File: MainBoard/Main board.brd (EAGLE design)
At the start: 100 x 80 mm, 9 parts

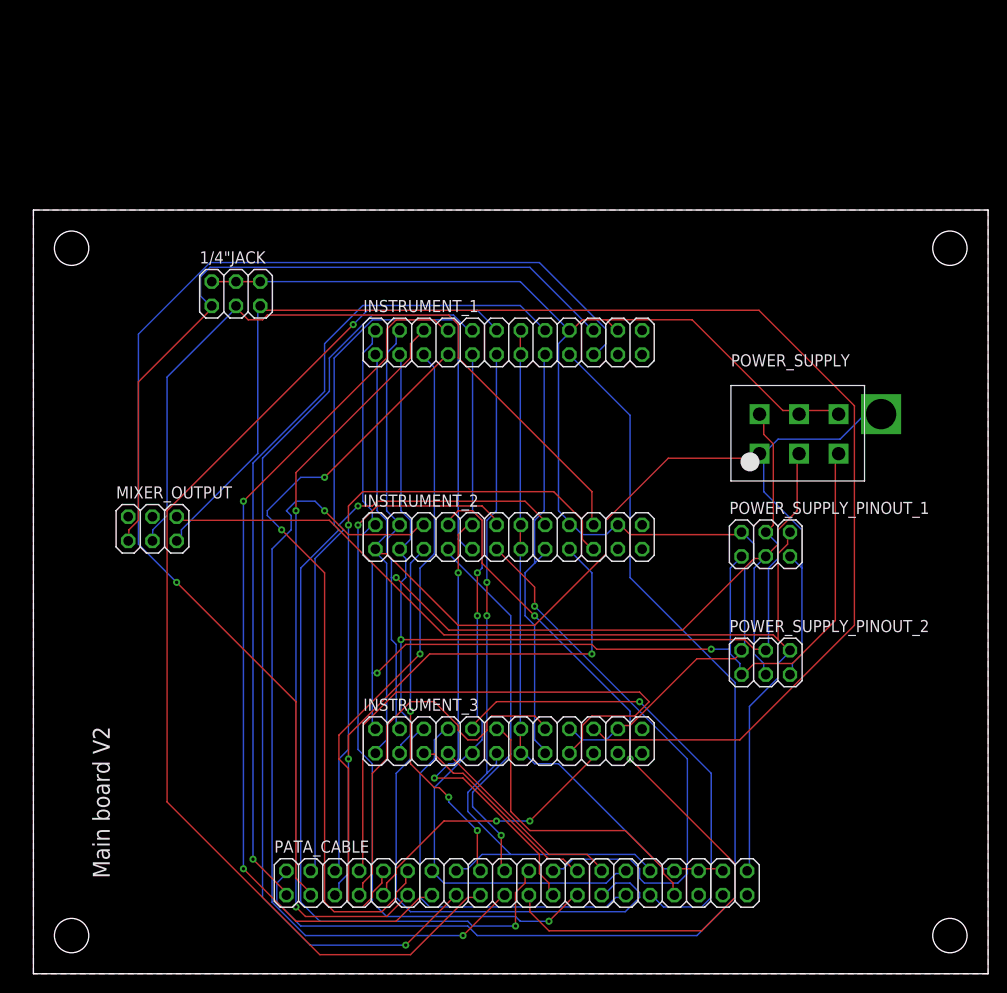
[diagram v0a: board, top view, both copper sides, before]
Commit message: Finished layout - needs silk screen
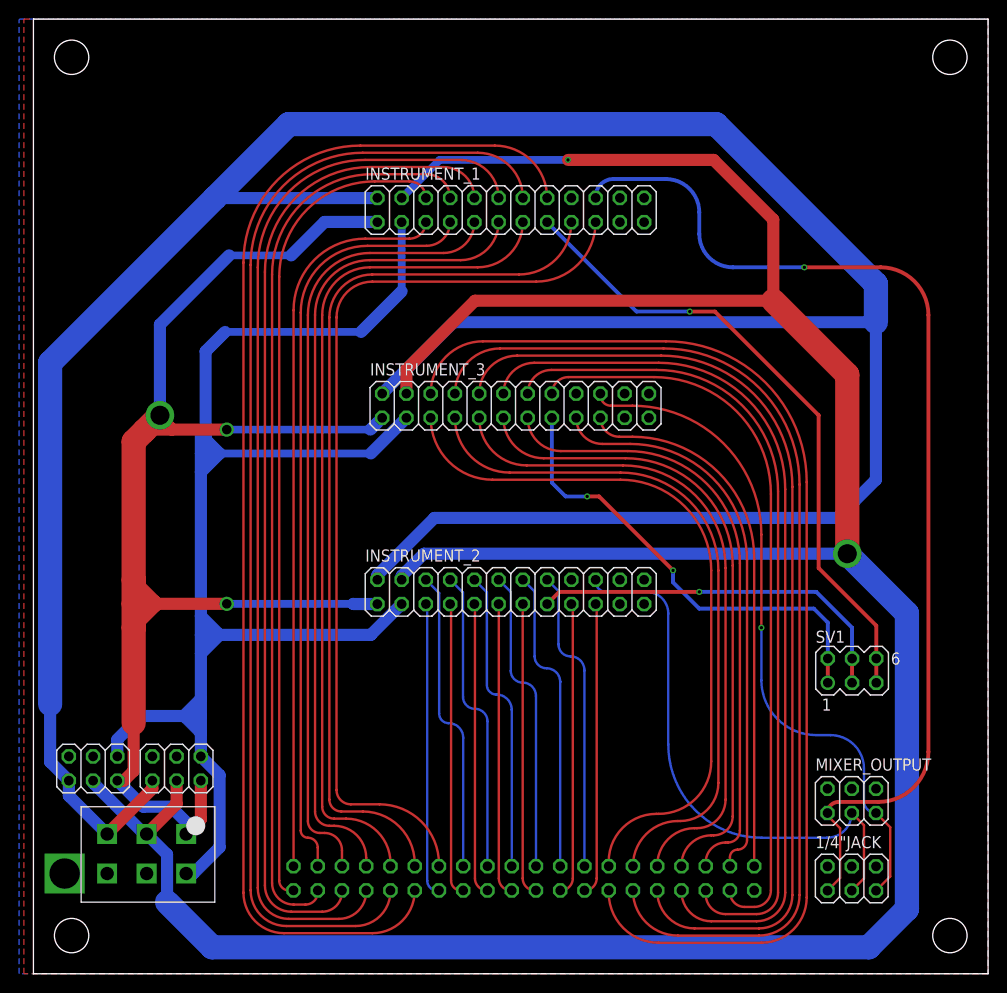
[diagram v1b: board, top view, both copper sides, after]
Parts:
- added SV1: (no value), con-lstb:MA03-2
- moved 1/4"JACK 88.9 mm to (85.7, 9.98)
- moved MIXER_OUTPUT 78.6 mm to (85.7, 18.1)
- moved POWER_SUPPLY 77.0 mm to (16.0, 10.5), turned to 180 degrees
- moved POWER_SUPPLY_PINOUT_1 74.3 mm to (6.25, 21.5)
- moved POWER_SUPPLY_PINOUT_2 62.7 mm to (15.0, 21.5)
- moved INSTRUMENT_3 35.1 mm to (50.5, 59.5)
- moved INSTRUMENT_1 13.9 mm to (50.0, 80.0)
- moved INSTRUMENT_2 5.75 mm to (50.0, 40.0)
- moved PATA_CABLE 0.89 mm to (51.4, 10.0), flipped to the bottom, turned to 180 degrees
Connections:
- net ANALOG_OUTPUT_1 renamed OUT1
- net ANALOG_OUTPUT_2 renamed OUT2
- net ANALOG_OUTPUT_3 renamed OUT3
- removed net ANALOG_GND: 1/4"JACK.2, 1/4"JACK.4, 1/4"JACK.6, INSTRUMENT_1.18, INSTRUMENT_1.22, INSTRUMENT_2.18, INSTRUMENT_2.22, INSTRUMENT_3.18, INSTRUMENT_3.22, POWER_SUPPLY.AGND0, POWER_SUPPLY.AGND1, POWER_SUPPLY_PINOUT_1.2, POWER_SUPPLY_PINOUT_2.2
- removed net DIGITAL_GND: INSTRUMENT_1.3, INSTRUMENT_2.3, INSTRUMENT_3.3, POWER_SUPPLY.DGND, POWER_SUPPLY_PINOUT_1.4, POWER_SUPPLY_PINOUT_2.4
- removed net GND: MIXER_OUTPUT.6, PATA_CABLE.40, POWER_SUPPLY_PINOUT_1.6, POWER_SUPPLY_PINOUT_2.6
- removed net SEQUENCER_TRIGGER: INSTRUMENT_1.15, INSTRUMENT_2.15, INSTRUMENT_3.15
- removed net SWITCH_2: INSTRUMENT_1.17, PATA_CABLE.2
- removed net SWITCH_3: INSTRUMENT_1.19, PATA_CABLE.3
- removed net SWITCH_4: INSTRUMENT_2.16, PATA_CABLE.4
- removed net SWITCH_5: INSTRUMENT_2.17, PATA_CABLE.5
- removed net SWITCH_6: INSTRUMENT_2.19, PATA_CABLE.6
- removed net SWITCH_7: INSTRUMENT_3.16, PATA_CABLE.7
- removed net SWITCH_8: INSTRUMENT_3.17, PATA_CABLE.8
- removed net SWITCH_9: INSTRUMENT_3.19, PATA_CABLE.9
- removed net TO_POT_PCB: INSTRUMENT_1.13, INSTRUMENT_1.14, INSTRUMENT_2.13, INSTRUMENT_2.14, INSTRUMENT_3.13, INSTRUMENT_3.14, PATA_CABLE.34, PATA_CABLE.36, PATA_CABLE.38
- new net AGND: 1/4"JACK.2, 1/4"JACK.4, 1/4"JACK.6, INSTRUMENT_1.18, INSTRUMENT_1.22, INSTRUMENT_2.18, INSTRUMENT_2.22, INSTRUMENT_3.18, INSTRUMENT_3.22, MIXER_OUTPUT.2, MIXER_OUTPUT.4, MIXER_OUTPUT.6, PATA_CABLE.40, POWER_SUPPLY.AGND0, POWER_SUPPLY.AGND1, POWER_SUPPLY_PINOUT_1.2, POWER_SUPPLY_PINOUT_1.4, POWER_SUPPLY_PINOUT_2.2, POWER_SUPPLY_PINOUT_2.4
- new net DGND: INSTRUMENT_1.3, INSTRUMENT_2.3, INSTRUMENT_3.3, POWER_SUPPLY.DGND, POWER_SUPPLY_PINOUT_1.6, POWER_SUPPLY_PINOUT_2.6
- new net POT_13A: INSTRUMENT_3.9, PATA_CABLE.31
- new net POT_13B: INSTRUMENT_3.10, PATA_CABLE.32
- new net POT_14A: INSTRUMENT_3.11, PATA_CABLE.33
- new net POT_14B: INSTRUMENT_3.12, PATA_CABLE.34
- new net POT_15A: INSTRUMENT_3.13, PATA_CABLE.35
- new net POT_15B: INSTRUMENT_3.14, PATA_CABLE.36
- new net POT_3A: INSTRUMENT_1.9, PATA_CABLE.5
- new net POT_4A: INSTRUMENT_1.11, PATA_CABLE.7
- new net SW_2: INSTRUMENT_1.17, PATA_CABLE.11
- new net SW_3: INSTRUMENT_1.19, PATA_CABLE.13
- new net SW_4: INSTRUMENT_2.16, PATA_CABLE.25
- new net SW_5: INSTRUMENT_2.17, PATA_CABLE.24
- new net SW_6: INSTRUMENT_2.19, PATA_CABLE.26
- new net SW_7: INSTRUMENT_3.16, PATA_CABLE.38
- new net SW_8: INSTRUMENT_3.17, PATA_CABLE.37
- new net SW_9: INSTRUMENT_3.19, PATA_CABLE.39
- new net TRIG1: INSTRUMENT_1.15, SV1.5, SV1.6
- new net TRIG2: INSTRUMENT_2.15, SV1.3, SV1.4
- new net TRIG3: INSTRUMENT_3.15, SV1.1, SV1.2
- net POT_10A: now also INSTRUMENT_2.13, PATA_CABLE.22; no longer INSTRUMENT_3.7, PATA_CABLE.28
- net POT_10B: now also INSTRUMENT_2.14, PATA_CABLE.23; no longer INSTRUMENT_3.8, PATA_CABLE.29
- net POT_11A: now also INSTRUMENT_3.5, PATA_CABLE.27; no longer INSTRUMENT_1.9, INSTRUMENT_3.9, PATA_CABLE.14, PATA_CABLE.30
- net POT_11B: now also INSTRUMENT_3.6, PATA_CABLE.28; no longer INSTRUMENT_3.10, PATA_CABLE.31
- net POT_12A: now also INSTRUMENT_3.7, PATA_CABLE.29; no longer INSTRUMENT_1.11, INSTRUMENT_3.11, PATA_CABLE.16, PATA_CABLE.32
- net POT_12B: now also INSTRUMENT_3.8, PATA_CABLE.30; no longer INSTRUMENT_3.12, PATA_CABLE.33
- net POT_1A: now also PATA_CABLE.1; no longer PATA_CABLE.10
- net POT_1B: now also PATA_CABLE.2; no longer PATA_CABLE.11
- net POT_2A: now also PATA_CABLE.3; no longer PATA_CABLE.12
- net POT_2B: now also PATA_CABLE.4; no longer PATA_CABLE.13
- net POT_3B: now also PATA_CABLE.6; no longer PATA_CABLE.15
- net POT_4B: now also PATA_CABLE.8; no longer PATA_CABLE.17
- net POT_5A: now also INSTRUMENT_1.13, PATA_CABLE.9; no longer INSTRUMENT_2.5, PATA_CABLE.18
- net POT_5B: now also INSTRUMENT_1.14, PATA_CABLE.10; no longer INSTRUMENT_2.6, PATA_CABLE.19
- net POT_6A: now also INSTRUMENT_2.5, PATA_CABLE.14; no longer INSTRUMENT_2.7, PATA_CABLE.20
- net POT_6B: now also INSTRUMENT_2.6, PATA_CABLE.15; no longer INSTRUMENT_2.8, PATA_CABLE.21
- net POT_7A: now also INSTRUMENT_2.7, PATA_CABLE.16; no longer INSTRUMENT_2.9, PATA_CABLE.22
- net POT_7B: now also INSTRUMENT_2.8, PATA_CABLE.17; no longer INSTRUMENT_2.10, PATA_CABLE.23
- net POT_8A: now also INSTRUMENT_2.9, PATA_CABLE.18; no longer INSTRUMENT_2.11, PATA_CABLE.24
- net POT_8B: now also INSTRUMENT_2.10, PATA_CABLE.19; no longer INSTRUMENT_2.12, PATA_CABLE.25
- net POT_9A: now also INSTRUMENT_2.11, PATA_CABLE.20; no longer INSTRUMENT_3.5, PATA_CABLE.26
- net POT_9B: now also INSTRUMENT_2.12, PATA_CABLE.21; no longer INSTRUMENT_3.6, PATA_CABLE.27
- net SWITCH_1: now also PATA_CABLE.12; no longer PATA_CABLE.1
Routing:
- net -12V: track 114.4 -> 317.3 mm, vias 1 -> 2
- net +12V: track 126.1 -> 312.4 mm, vias 2 -> 0
- net DGND: track 0.00 -> 160.7 mm
- net ANALOG_GND: track 151.1 -> 0.00 mm
- net SWITCH_3: track 124.5 -> 0.00 mm, vias 1 -> 0
- net SWITCH_2: track 118.9 -> 0.00 mm
- net DIGITAL_GND: track 109.7 -> 0.00 mm, vias 1 -> 0
- net GND: track 106.7 -> 0.00 mm
- net POT_13B: track 0.00 -> 100.2 mm
- net POT_7A: track 128.1 -> 30.7 mm, vias 1 -> 0
- net SW_3: track 0.00 -> 95.0 mm
- net POT_14B: track 0.00 -> 92.1 mm
- net SW_2: track 0.00 -> 92.0 mm
- net POT_15B: track 0.00 -> 84.3 mm
- net POT_4A: track 0.00 -> 83.5 mm
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- added copper zone on layer 1, net AGND
- added copper zone on layer 16, net AGND
- removed copper zone on layer 1, net GND
- removed copper zone on layer 16, net GND
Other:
- board size 100 x 80 mm -> 100 x 100 mm
- board text removed: "Main board V2"
